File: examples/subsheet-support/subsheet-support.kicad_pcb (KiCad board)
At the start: 2 copper layers, 4 parts

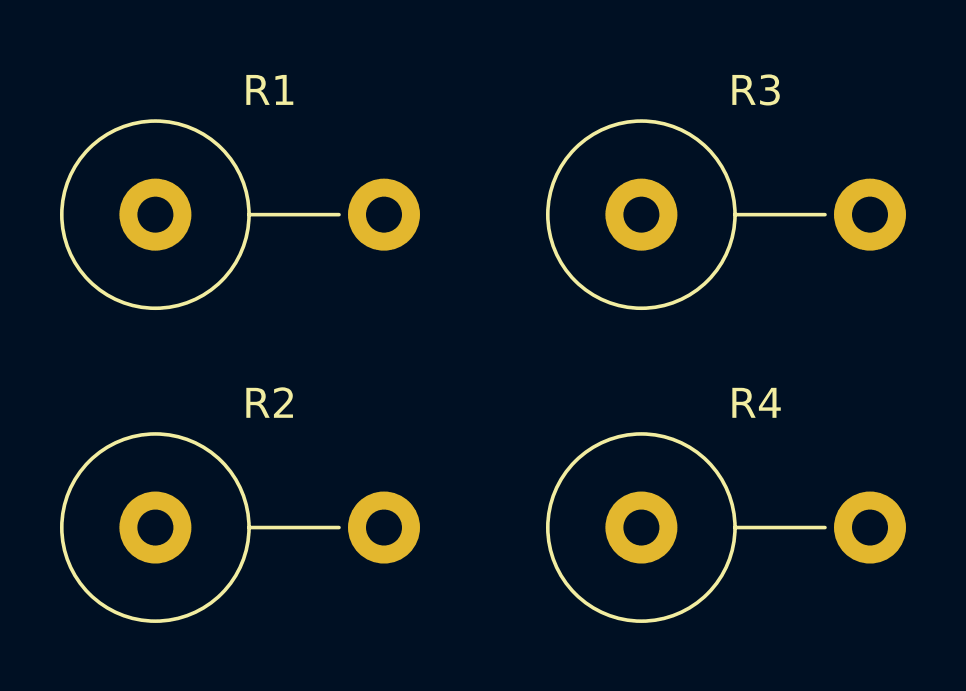
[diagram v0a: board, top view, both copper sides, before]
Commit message: Improved test coverage.
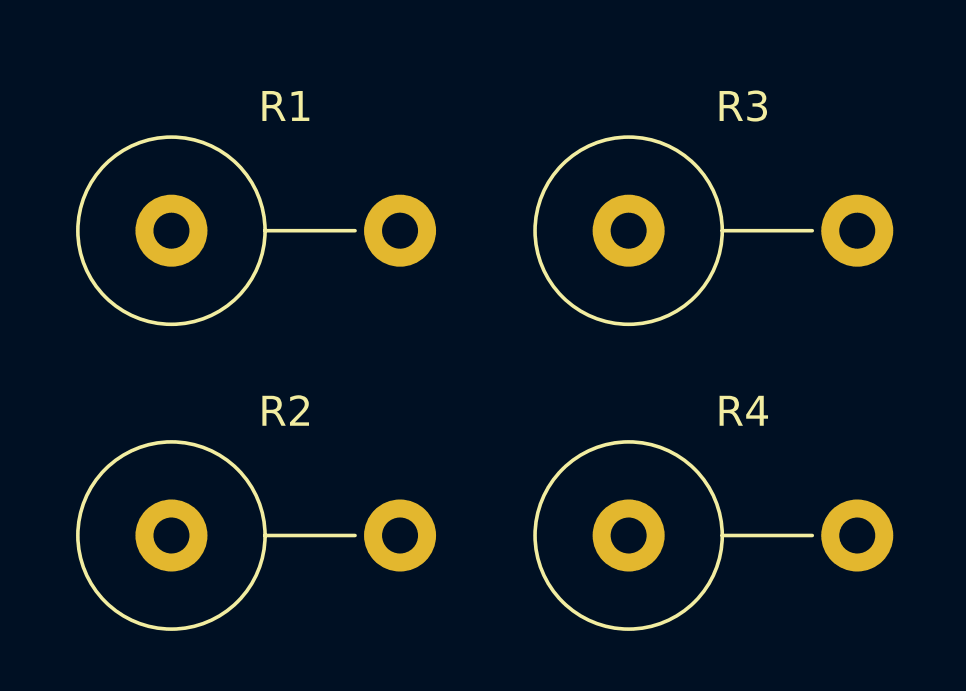
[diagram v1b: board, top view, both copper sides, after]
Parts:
- moved R1 0.76 mm to (105.4, 69.8)
- moved R3 0.68 mm to (120.7, 69.8)
- moved R2 0.60 mm to (105.4, 80.0)
- moved R4 0.50 mm to (120.7, 80.0)
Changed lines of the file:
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@@
     (pad_to_mask_clearance 0.2)
     (aux_axis_origin 0 0)
-    (visible_elements FFFFFF7F)
+    (visible_elements 7FFFFFFF)
     (pcbplotparams
       (layerselection 0x010fc_ffffffff)
@@
   )
   (module Resistor_THT:R_Axial_DIN0617_L17.0mm_D6.0mm_P7.62mm_Vertical (layer F.Cu)
-    (at 121.075001 79.745001)
+    (at 120.65 80.01)
     (descr "Resistor, Axial_DIN0617 series, Axial, Vertical, pin pitch=7.62mm, 2W, length*diameter=17*6mm^2, http://www.vishay.com/docs/20128/wkxwrx.pdf")
     (tags "Resistor Axial_DIN0617 series Axial Vertical pin pitch 7.62mm 2W length 17mm diameter 6mm")
@@
   )
   (module Resistor_THT:R_Axial_DIN0617_L17.0mm_D6.0mm_P7.62mm_Vertical (layer F.Cu)
-    (at 121.075001 69.315001)
+    (at 120.65 69.85)
     (descr "Resistor, Axial_DIN0617 series, Axial, Vertical, pin pitch=7.62mm, 2W, length*diameter=17*6mm^2, http://www.vishay.com/docs/20128/wkxwrx.pdf")
     (tags "Resistor Axial_DIN0617 series Axial Vertical pin pitch 7.62mm 2W length 17mm diameter 6mm")
@@
   )
   (module Resistor_THT:R_Axial_DIN0617_L17.0mm_D6.0mm_P7.62mm_Vertical (layer F.Cu)
-    (at 104.875001 79.745001)
+    (at 105.41 80.01)
     (descr "Resistor, Axial_DIN0617 series, Axial, Vertical, pin pitch=7.62mm, 2W, length*diameter=17*6mm^2, http://www.vishay.com/docs/20128/wkxwrx.pdf")
     (tags "Resistor Axial_DIN0617 series Axial Vertical pin pitch 7.62mm 2W length 17mm diameter 6mm")
@@
   )
   (module Resistor_THT:R_Axial_DIN0617_L17.0mm_D6.0mm_P7.62mm_Vertical (layer F.Cu)
-    (at 104.875001 69.315001)
+    (at 105.41 69.85)
     (descr "Resistor, Axial_DIN0617 series, Axial, Vertical, pin pitch=7.62mm, 2W, length*diameter=17*6mm^2, http://www.vishay.com/docs/20128/wkxwrx.pdf")
     (tags "Resistor Axial_DIN0617 series Axial Vertical pin pitch 7.62mm 2W length 17mm diameter 6mm")
